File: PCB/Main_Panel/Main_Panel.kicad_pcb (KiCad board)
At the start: 2 copper layers, 170 x 170 mm, 3 parts, among them IC1 TCA6424ARGJR, U1 Pico, U2 TLC5947DAP

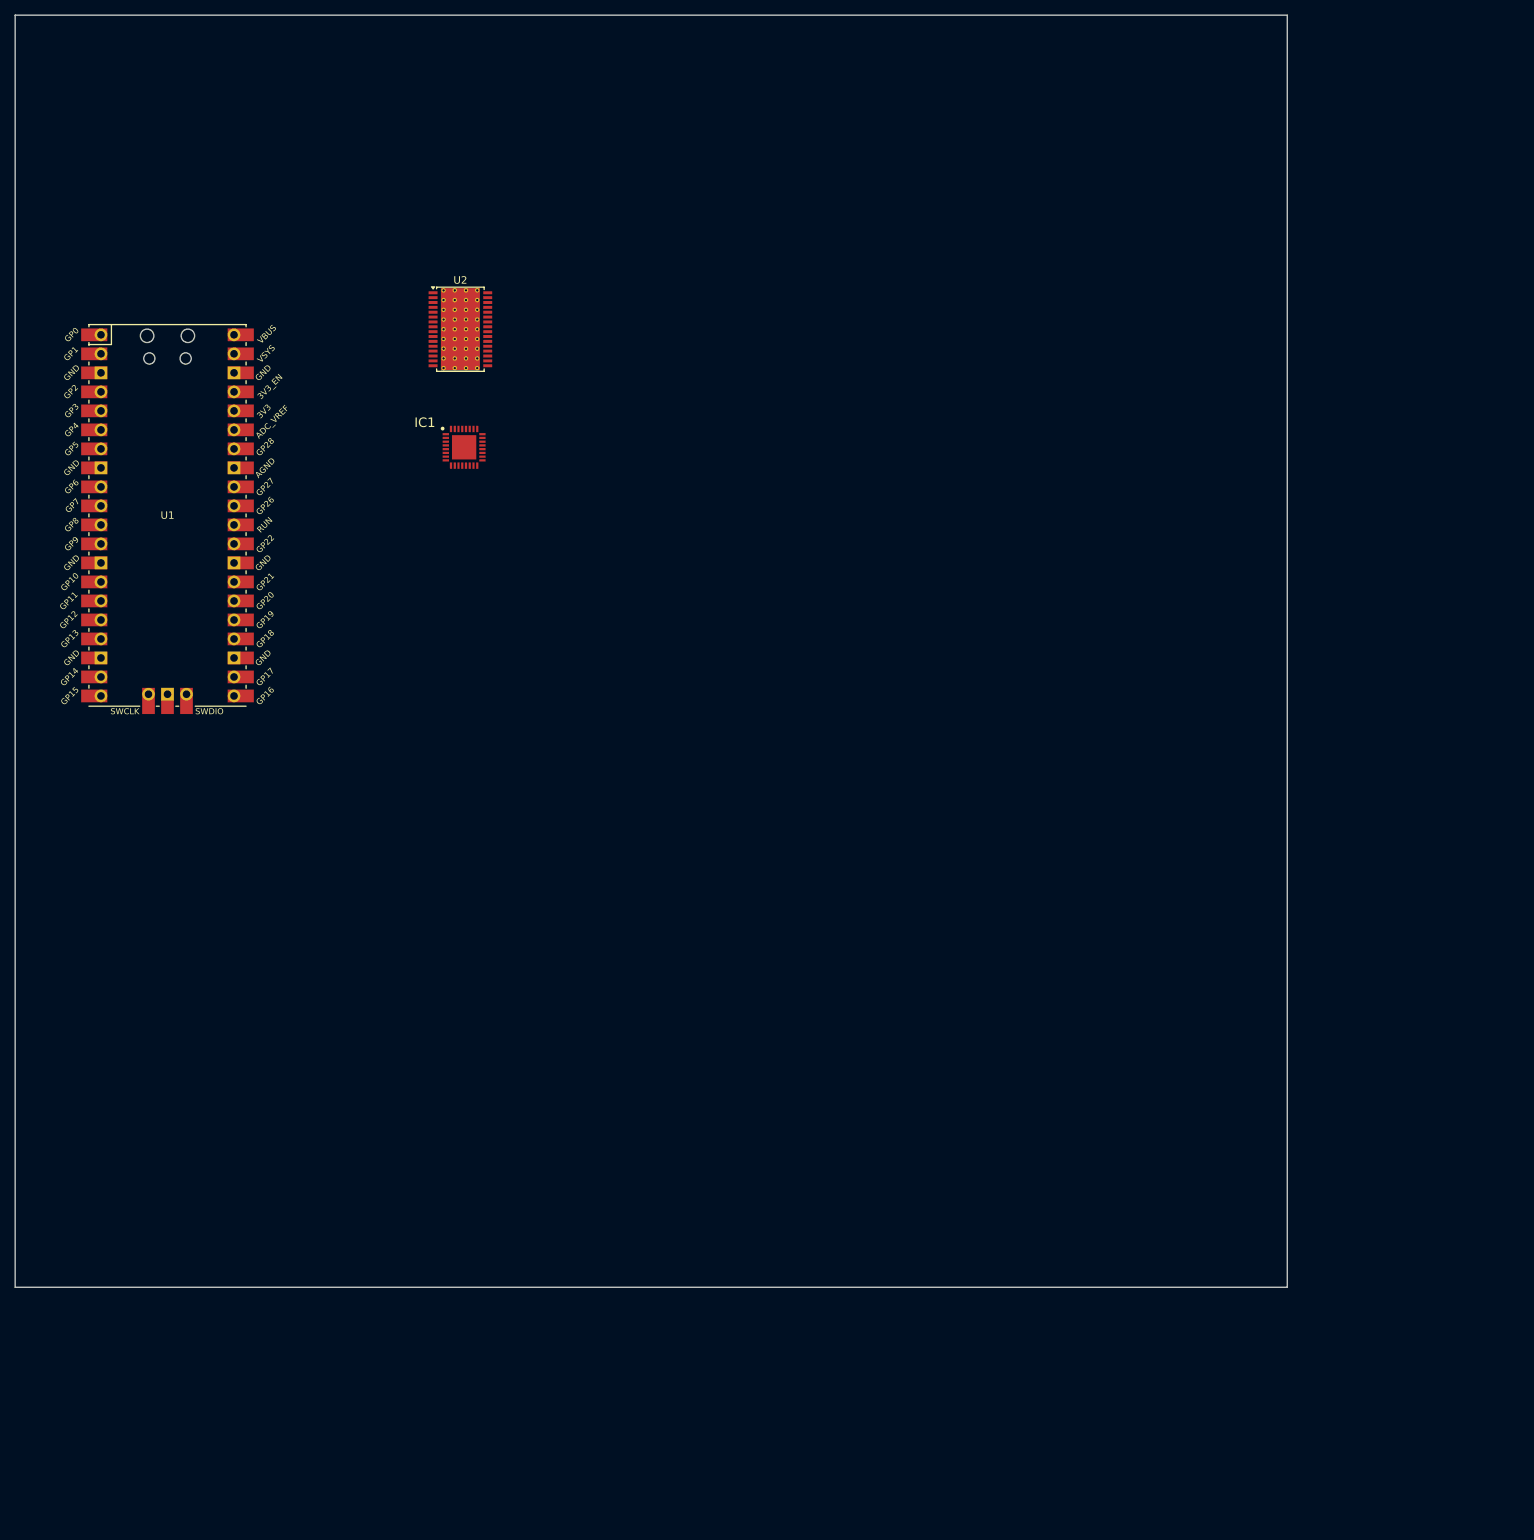
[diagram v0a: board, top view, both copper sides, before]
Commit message: PCB Designs
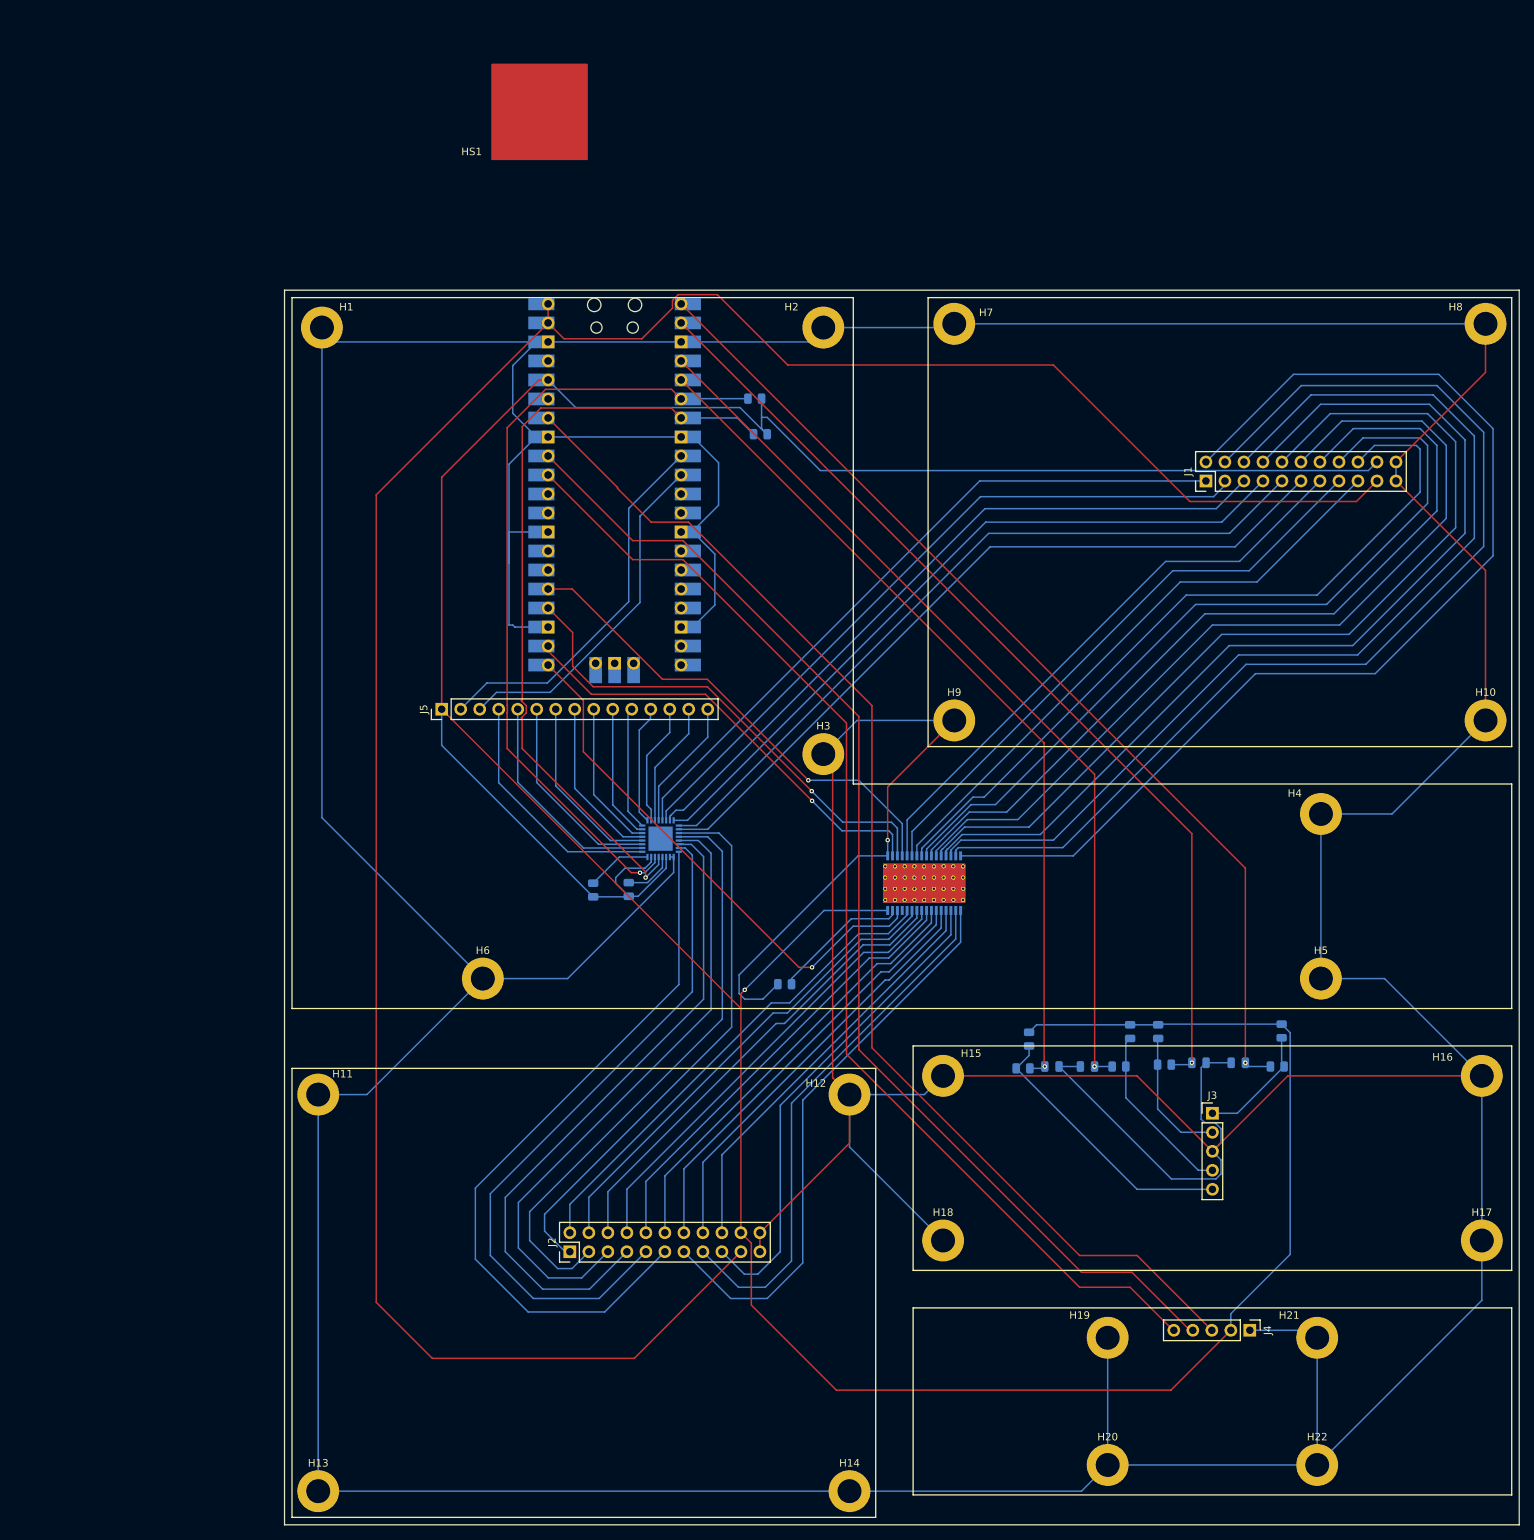
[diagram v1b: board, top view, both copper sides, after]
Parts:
- added C1: 0.01uF, Capacitor_SMD:C_0805_2012Metric, B.Cu at (167.3, 163.8)
- added C2: 0.01uF, Capacitor_SMD:C_0805_2012Metric, B.Cu at (162.6, 163.8)
- added C3: 0.01uF, Capacitor_SMD:C_0805_2012Metric, B.Cu at (187.4, 163.2)
- added C4: 0.01uF, Capacitor_SMD:C_0805_2012Metric, B.Cu at (182.2, 163.2)
- added H1: MountingHole_Pad, MountingHole:MountingHole_3.2mm_M3_DIN965_Pad, F.Cu at (65.0, 65.0)
- added H10: MountingHole_Pad, MountingHole:MountingHole_3.2mm_M3_DIN965_Pad, F.Cu at (220.5, 117.5)
- added H11: MountingHole_Pad, MountingHole:MountingHole_3.2mm_M3_DIN965_Pad, F.Cu at (64.5, 167.5)
- added H12: MountingHole_Pad, MountingHole:MountingHole_3.2mm_M3_DIN965_Pad, F.Cu at (135.5, 167.5)
- added H13: MountingHole_Pad, MountingHole:MountingHole_3.2mm_M3_DIN965_Pad, F.Cu at (64.5, 220.5)
- added H14: MountingHole_Pad, MountingHole:MountingHole_3.2mm_M3_DIN965_Pad, F.Cu at (135.5, 220.5)
- added H15: MountingHole_Pad, MountingHole:MountingHole_3.2mm_M3_DIN965_Pad, F.Cu at (148.0, 165.0)
- added H16: MountingHole_Pad, MountingHole:MountingHole_3.2mm_M3_DIN965_Pad, F.Cu at (220.0, 165.0)
- added H17: MountingHole_Pad, MountingHole:MountingHole_3.2mm_M3_DIN965_Pad, F.Cu at (220.0, 187.0)
- added H18: MountingHole_Pad, MountingHole:MountingHole_3.2mm_M3_DIN965_Pad, F.Cu at (148.0, 187.0)
- added H19: MountingHole_Pad, MountingHole:MountingHole_3.2mm_M3_DIN965_Pad, F.Cu at (170.0, 200.0)
- added H2: MountingHole_Pad, MountingHole:MountingHole_3.2mm_M3_DIN965_Pad, F.Cu at (132.0, 65.0)
- added H20: MountingHole_Pad, MountingHole:MountingHole_3.2mm_M3_DIN965_Pad, F.Cu at (170.0, 217.0)
- added H21: MountingHole_Pad, MountingHole:MountingHole_3.2mm_M3_DIN965_Pad, F.Cu at (198.0, 200.0)
- added H22: MountingHole_Pad, MountingHole:MountingHole_3.2mm_M3_DIN965_Pad, F.Cu at (198.0, 217.0)
- added H3: MountingHole_Pad, MountingHole:MountingHole_3.2mm_M3_DIN965_Pad, F.Cu at (132.0, 122.0)
- added H4: MountingHole_Pad, MountingHole:MountingHole_3.2mm_M3_DIN965_Pad, F.Cu at (198.5, 130.0)
- added H5: MountingHole_Pad, MountingHole:MountingHole_3.2mm_M3_DIN965_Pad, F.Cu at (198.5, 152.0)
- added H6: MountingHole_Pad, MountingHole:MountingHole_3.2mm_M3_DIN965_Pad, F.Cu at (86.5, 152.0)
- added H7: MountingHole_Pad, MountingHole:MountingHole_3.2mm_M3_DIN965_Pad, F.Cu at (149.5, 64.5)
- added H8: MountingHole_Pad, MountingHole:MountingHole_3.2mm_M3_DIN965_Pad, F.Cu at (220.5, 64.5)
- added H9: MountingHole_Pad, MountingHole:MountingHole_3.2mm_M3_DIN965_Pad, F.Cu at (149.5, 117.5)
- added HS1: Heatsink_Pad, Control_Panel_Footprints:Heat Sink, F.Cu at (87.7, 42.5)
- added J1: Conn_02x11_Odd_Even, Connector_PinHeader_2.54mm:PinHeader_2x11_P2.54mm_Vertical, F.Cu at (183.1, 85.5)
- added J2: Conn_02x11_Odd_Even, Connector_PinHeader_2.54mm:PinHeader_2x11_P2.54mm_Vertical, F.Cu at (98.1, 188.5)
- added J3: Conn_01x05, Connector_PinHeader_2.54mm:PinHeader_1x05_P2.54mm_Vertical, F.Cu at (184.0, 170.0)
- added J4: Conn_01x05, Connector_PinHeader_2.54mm:PinHeader_1x05_P2.54mm_Vertical, F.Cu at (189.0, 199.0)
- added J5: Conn_01x15, Connector_PinHeader_2.54mm:PinHeader_1x15_P2.54mm_Vertical, F.Cu at (81.0, 116.0)
- added R1: 10k, Resistor_SMD:R_0805_2012Metric, B.Cu at (106.0, 140.1)
- added R2: 10k, Resistor_SMD:R_0805_2012Metric, B.Cu at (123.6, 79.2)
- added R3: 10k, Resistor_SMD:R_0805_2012Metric, B.Cu at (122.8, 74.5)
- added R30: 10k, Resistor_SMD:R_0805_2012Metric, B.Cu at (159.5, 160.1)
- added R31: 10k, Resistor_SMD:R_0805_2012Metric, B.Cu at (171.5, 163.8)
- added R32: 10k, Resistor_SMD:R_0805_2012Metric, B.Cu at (173.0, 159.1)
- added R33: 10k, Resistor_SMD:R_0805_2012Metric, B.Cu at (158.7, 164.0)
- added R34: 10k, Resistor_SMD:R_0805_2012Metric, B.Cu at (193.2, 159.0)
- added R35: 10k, Resistor_SMD:R_0805_2012Metric, B.Cu at (176.8, 159.1)
- added R36: 10k, Resistor_SMD:R_0805_2012Metric, B.Cu at (192.7, 163.8)
- added R37: 10k, Resistor_SMD:R_0805_2012Metric, B.Cu at (177.6, 163.5)
- added R4: 10k, Resistor_SMD:R_0805_2012Metric, B.Cu at (101.2, 140.2)
- added R5: 2460, Resistor_SMD:R_0805_2012Metric, B.Cu at (126.8, 152.8)
- IC1, U1, U2: moved to B.Cu
- moved U2 96.5 mm to (145.5, 139.2), turned to -90 degrees
- moved U1 59.9 mm to (104.1, 86.0), turned to 180 degrees
- moved IC1 58.5 mm to (110.2, 133.3)
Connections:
- IC1 pad 1: unconnected-(IC1-P00-Pad1) -> /Switch2
- IC1 pad 10: unconnected-(IC1-P11-Pad10) -> /Switch11
- IC1 pad 11: unconnected-(IC1-P12-Pad11) -> /Switch12
- IC1 pad 12: unconnected-(IC1-P13-Pad12) -> /Switch13
- IC1 pad 13: unconnected-(IC1-P14-Pad13) -> /Button0
- IC1 pad 14: unconnected-(IC1-P15-Pad14) -> /Button1
- IC1 pad 15: unconnected-(IC1-P16-Pad15) -> /Button2
- IC1 pad 16: unconnected-(IC1-P17-Pad16) -> /Button3
- IC1 pad 17: unconnected-(IC1-P20-Pad17) -> /Button4
- IC1 pad 18: unconnected-(IC1-P21-Pad18) -> /Button5
- IC1 pad 19: unconnected-(IC1-P22-Pad19) -> /Button6
- IC1 pad 2: unconnected-(IC1-P01-Pad2) -> /Switch3
- IC1 pad 20: unconnected-(IC1-P23-Pad20) -> /Button7
- IC1 pad 21: unconnected-(IC1-P24-Pad21) -> /Button8
- IC1 pad 22: unconnected-(IC1-P25-Pad22) -> /Button9
- IC1 pad 23: unconnected-(IC1-P26-Pad23) -> /Button10
- IC1 pad 24: unconnected-(IC1-P27-Pad24) -> /Button11
- IC1 pad 25: unconnected-(IC1-GND-Pad25) -> GND
- IC1 pad 26: unconnected-(IC1-ADDR-Pad26) -> GND
- IC1 pad 27: unconnected-(IC1-V_CCP-Pad27) -> +3.3V
- IC1 pad 28: unconnected-(IC1-~{RESET}-Pad28) -> Net-(IC1-~{RESET})
- IC1 pad 29: unconnected-(IC1-SCL-Pad29) -> SCL
- IC1 pad 3: unconnected-(IC1-P02-Pad3) -> /Switch4
- IC1 pad 30: unconnected-(IC1-SDA-Pad30) -> SDA
- IC1 pad 31: unconnected-(IC1-V_CCI-Pad31) -> +3.3V
- IC1 pad 32: unconnected-(IC1-~{INT}-Pad32) -> Net-(IC1-~{INT})
- IC1 pad 4: unconnected-(IC1-P03-Pad4) -> /Switch5
- IC1 pad 5: unconnected-(IC1-P04-Pad5) -> /Switch6
- IC1 pad 6: unconnected-(IC1-P05-Pad6) -> /Switch7
- IC1 pad 7: unconnected-(IC1-P06-Pad7) -> /Switch8
- IC1 pad 8: unconnected-(IC1-P07-Pad8) -> /Switch9
- IC1 pad 9: unconnected-(IC1-P10-Pad9) -> /Switch10
- U1 pad 1: unconnected-(U1-GPIO0-Pad1) -> /Encoder_0_B
- U1 pad 10: unconnected-(U1-GPIO7-Pad10) -> /Switch1
- U1 pad 13: unconnected-(U1-GND-Pad13) -> GND
- U1 pad 18: unconnected-(U1-GND-Pad18) -> GND
- U1 pad 2: unconnected-(U1-GPIO1-Pad2) -> /Encoder_0_A
- U1 pad 21: unconnected-(U1-GPIO16-Pad21) -> XLAT
- U1 pad 22: unconnected-(U1-GPIO17-Pad22) -> Blank
- U1 pad 23: unconnected-(U1-GND-Pad23) -> GND
- U1 pad 24: unconnected-(U1-GPIO18-Pad24) -> SCK
- U1 pad 25: unconnected-(U1-GPIO19-Pad25) -> MOSI
- U1 pad 28: unconnected-(U1-GND-Pad28) -> GND
- U1 pad 3: unconnected-(U1-GND-Pad3) -> GND
- U1 pad 31: unconnected-(U1-GPIO26_ADC0-Pad31) -> /Pot2
- U1 pad 32: unconnected-(U1-GPIO27_ADC1-Pad32) -> /Pot1
- U1 pad 33: unconnected-(U1-AGND-Pad33) -> GND
- U1 pad 34: unconnected-(U1-GPIO28_ADC2-Pad34) -> /Pot0
- U1 pad 36: unconnected-(U1-3V3-Pad36) -> +3.3V
- U1 pad 38: unconnected-(U1-GND-Pad38) -> GND
- U1 pad 39: unconnected-(U1-VSYS-Pad39) -> +5V
- U1 pad 4: unconnected-(U1-GPIO2-Pad4) -> /Encoder_1_B
- U1 pad 40: unconnected-(U1-VBUS-Pad40) -> +5V
- U1 pad 5: unconnected-(U1-GPIO3-Pad5) -> /Encoder_1_A
- U1 pad 6: unconnected-(U1-GPIO4-Pad6) -> SDA
- U1 pad 7: unconnected-(U1-GPIO5-Pad7) -> SCL
- U1 pad 8: unconnected-(U1-GND-Pad8) -> GND
- U1 pad 9: unconnected-(U1-GPIO6-Pad9) -> /Switch0
- U2 pad 1: unconnected-(U2-GND-Pad1) -> GND
- U2 pad 10: unconnected-(U2-OUT5-Pad10) -> /LED9
- U2 pad 11: unconnected-(U2-OUT6-Pad11) -> /LED8
- U2 pad 12: unconnected-(U2-OUT7-Pad12) -> /LED7
- U2 pad 13: unconnected-(U2-OUT8-Pad13) -> /LED6
- U2 pad 14: unconnected-(U2-OUT9-Pad14) -> /LED5
- U2 pad 15: unconnected-(U2-OUT10-Pad15) -> /LED4
- U2 pad 16: unconnected-(U2-OUT11-Pad16) -> /LED3
- U2 pad 17: unconnected-(U2-OUT12-Pad17) -> /LED12
- U2 pad 18: unconnected-(U2-OUT13-Pad18) -> /LED13
- U2 pad 19: unconnected-(U2-OUT14-Pad19) -> /LED14
- U2 pad 2: unconnected-(U2-BLANK-Pad2) -> Blank
- U2 pad 20: unconnected-(U2-OUT15-Pad20) -> /LED23
- U2 pad 21: unconnected-(U2-OUT16-Pad21) -> /LED22
- U2 pad 22: unconnected-(U2-OUT17-Pad22) -> /LED21
- U2 pad 23: unconnected-(U2-OUT18-Pad23) -> /LED20
- U2 pad 24: unconnected-(U2-OUT19-Pad24) -> /LED19
- U2 pad 25: unconnected-(U2-OUT20-Pad25) -> /LED18
- U2 pad 26: unconnected-(U2-OUT21-Pad26) -> /LED17
- U2 pad 27: unconnected-(U2-OUT22-Pad27) -> /LED16
- U2 pad 28: unconnected-(U2-OUT23-Pad28) -> /LED15
- U2 pad 3: unconnected-(U2-SCLK-Pad3) -> SCK
- U2 pad 30: unconnected-(U2-XLAT-Pad30) -> XLAT
- U2 pad 31: unconnected-(U2-IREF-Pad31) -> Net-(U2-IREF)
- U2 pad 32: unconnected-(U2-VCC-Pad32) -> +3.3V
- U2 pad 33: unconnected-(U2-PowerPAD-Pad33) -> Net-(U2-PowerPAD)
- U2 pad 4: unconnected-(U2-SIN-Pad4) -> MOSI
- U2 pad 5: unconnected-(U2-OUT0-Pad5) -> /LED0
- U2 pad 6: unconnected-(U2-OUT1-Pad6) -> /LED1
- U2 pad 7: unconnected-(U2-OUT2-Pad7) -> /LED2
- U2 pad 8: unconnected-(U2-OUT3-Pad8) -> /LED11
- U2 pad 9: unconnected-(U2-OUT4-Pad9) -> /LED10
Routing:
- net GND: track 0.00 -> 1168.7 mm, vias 0 -> 1
- net +3.3V: track 0.00 -> 502.5 mm, vias 0 -> 1
- net +5V: track 0.00 -> 328.0 mm
- net /Pot0: track 0.00 -> 166.1 mm
- net /Pot1: track 0.00 -> 160.6 mm
- net /Pot2: track 0.00 -> 156.9 mm
- net /LED3: track 0.00 -> 151.0 mm
- net /LED4: track 0.00 -> 144.8 mm
- net /LED5: track 0.00 -> 138.4 mm
- net /Encoder_0_B: track 0.00 -> 136.2 mm, vias 0 -> 1
- net /LED6: track 0.00 -> 132.3 mm
- net /Encoder_0_A: track 0.00 -> 129.6 mm, vias 0 -> 1
- net /LED7: track 0.00 -> 126.3 mm
- net /LED8: track 0.00 -> 120.0 mm
- net /Encoder_1_B: track 0.00 -> 119.5 mm, vias 0 -> 1
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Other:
- board size 170 x 170 mm -> 165 x 165 mm
